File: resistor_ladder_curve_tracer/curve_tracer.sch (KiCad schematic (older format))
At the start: 7 parts, among them J2 Conn_01x10_Female, J3 Conn_01x10_Female

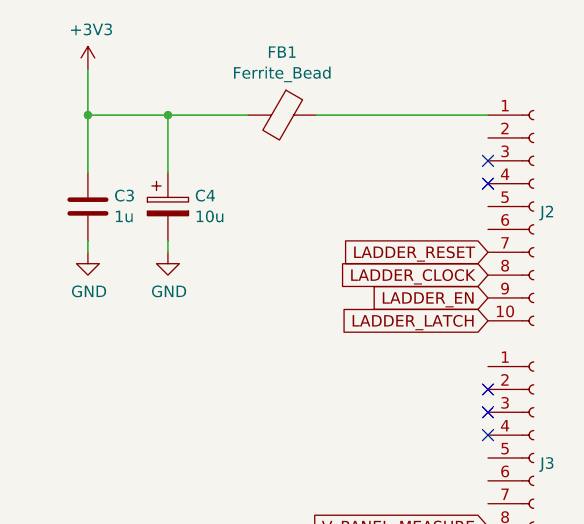
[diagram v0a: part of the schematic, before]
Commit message: Working on NREL pieces
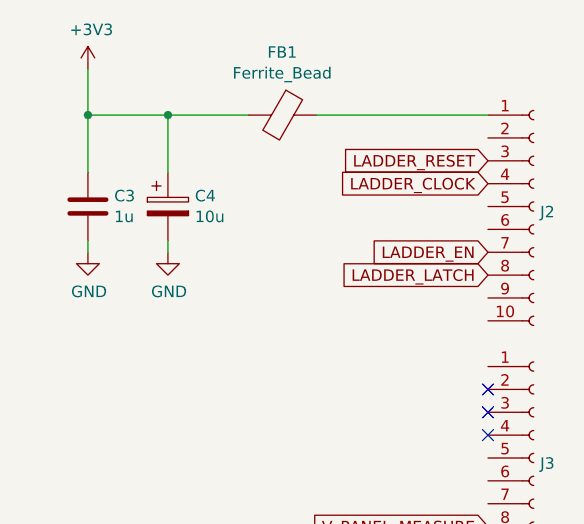
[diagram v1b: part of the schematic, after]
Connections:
- net LADDER_CLOCK: now also J2.4 (Pin_4); no longer J2.8 (Pin_8)
- net LADDER_EN: now also J2.7 (Pin_7); no longer J2.9 (Pin_9)
- net LADDER_LATCH: now also J2.8 (Pin_8); no longer J2.10 (Pin_10)
- net LADDER_RESET: now also J2.3 (Pin_3); no longer J2.7 (Pin_7)
- no-connect marks 5 -> 3
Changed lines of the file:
@@
 Text GLabel 9100 4900 0    50   Input ~ 0
 V_PANEL_MEASURE
-Text GLabel 9100 3900 0    50   Input ~ 0
+Text GLabel 9100 3700 0    50   Input ~ 0
 LADDER_EN
-Text GLabel 9100 3800 0    50   Input ~ 0
+Text GLabel 9100 3400 0    50   Input ~ 0
 LADDER_CLOCK
-Text GLabel 9100 3700 0    50   Input ~ 0
+Text GLabel 9100 3300 0    50   Input ~ 0
 LADDER_RESET
 $Comp
@@
 Wire Wire Line
 	9000 5100 9000 5200
-NoConn ~ 9100 3300
-NoConn ~ 9100 3400
 NoConn ~ 9100 4300
 NoConn ~ 9100 4400
@@
 Wire Wire Line
 	6250 4250 5100 4250
-Text GLabel 9100 4000 0    50   Input ~ 0
+Text GLabel 9100 3800 0    50   Input ~ 0
 LADDER_LATCH
 Wire Wire Line
